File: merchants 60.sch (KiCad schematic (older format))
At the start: 182 parts, among them SW1 SW_PUSH, U1 ATmega32U4-AU, Y1 16MHz

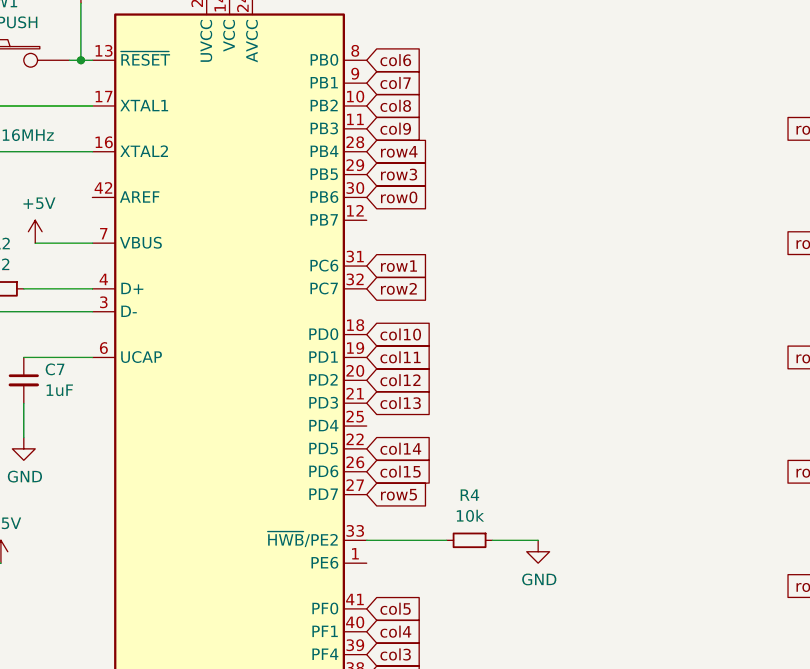
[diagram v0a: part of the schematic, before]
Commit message: Minor Changes
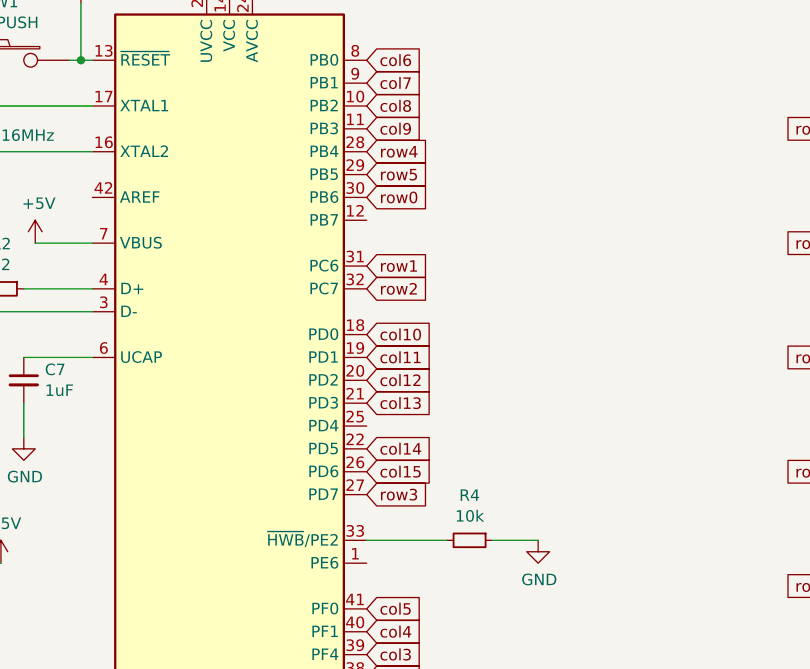
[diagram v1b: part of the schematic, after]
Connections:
- net row3: now also U1.27 (PD7); no longer U1.29 (PB5)
- net row5: now also U1.29 (PB5); no longer U1.27 (PD7)
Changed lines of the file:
@@
 row2
 Text GLabel 7550 2600 2    50   Input ~ 0
-row3
-Text GLabel 7550 2500 2    50   Input ~ 0
-row4
-Text GLabel 7550 4000 2    50   Input ~ 0
 row5
 Connection ~ 6850 5400
@@
 Text GLabel 7550 3900 2    50   Input ~ 0
 col15
-Text GLabel 7550 4500 2    50   Input ~ 0
-col5
 Text GLabel 7550 4600 2    50   Input ~ 0
 col4
@@
 Text GLabel 7550 4900 2    50   Input ~ 0
 col1
+Text GLabel 7550 4000 2    50   Input ~ 0
+row3
+Text GLabel 7550 2500 2    50   Input ~ 0
+row4
+Text GLabel 7550 4500 2    50   Input ~ 0
+col5
 $EndSCHEMATC

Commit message: Minor Changes
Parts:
- SW1: symbol keyboard_parts:SW_PUSH -> merchants-60-rescue:SW_PUSH-keyboard_parts
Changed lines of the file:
@@
 	5600 2650 5600 2400
 $Comp
-L keyboard_parts:SW_PUSH SW1
+L merchants-60-rescue:SW_PUSH-keyboard_parts SW1
 U 1 1 5F720C2E
 P 5950 2100
